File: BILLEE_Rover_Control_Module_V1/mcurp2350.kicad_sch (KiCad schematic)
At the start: 53 parts, among them CN14 DF11-18DP-2DSA, J1 2.54mm Header, SW2 KMR2, SW3 RESET SW, U15 W25Q128JVSIQTR, U16 SN74LVC244APWR, U17 ABM8-272-T3_C20625731, U18 RP2350A_C42411118, U21 TCA4307DGKR, U22 TCA4307DGKR

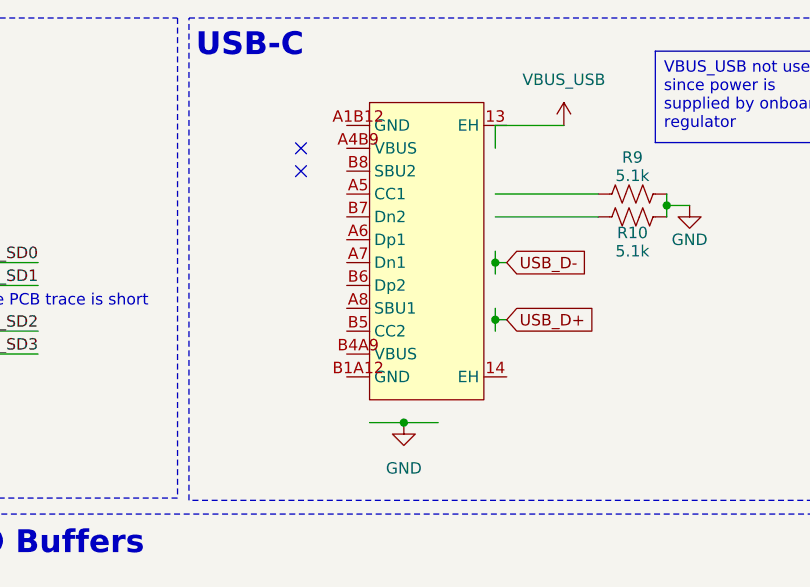
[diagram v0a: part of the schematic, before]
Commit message: Updated for schematic review by claude
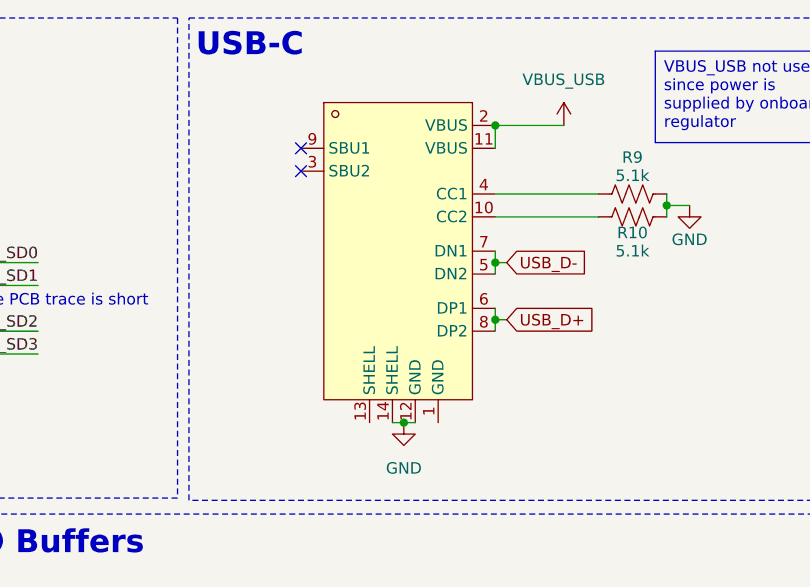
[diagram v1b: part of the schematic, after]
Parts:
- removed USB1: TYPE-C 16PIN 2MD, PDB_LCSC:USB-C-SMD_TYPE-C-16PIN-2MD-073, symbol PDB_LCSC_Libs:TYPE-C16PIN2MD
- added USB2: TYPE-C 16PIN 2MD, PDB_LCSC:USB-C-SMD_TYPE-C-16PIN-2MD-073, symbol PDB_LCSC_Libs:TYPE-C16PIN2MD
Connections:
- net GND: now also USB2.12 (GND), USB2.14 (SHELL)
- net USB_D+: now also USB2.6 (DP1), USB2.8 (DP2)
- net USB_D-: now also USB2.5 (DN2), USB2.7 (DN1)
- net VBUS_USB: now also USB2.11 (VBUS), USB2.2 (VBUS)
- net at R9.1: now also USB2.4 (CC1)
- net at R10.1: now also USB2.10 (CC2)
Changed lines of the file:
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@@
 	)
 	(junction
+		(at 363.22 26.67)
+		(diameter 0)
+		(color 0 0 0 0)
+	)
+	(junction
 		(at 99.06 46.99)
 		(diameter 0)
@@
 	(wire
 		(pts
-			(xy 353.06 59.69) (xy 356.87 59.69)
+			(xy 353.06 59.69) (xy 354.33 59.69)
 		)
 		(stroke
@@
 	(wire
 		(pts
+			(xy 351.79 59.69) (xy 353.06 59.69)
+		)
+		(stroke
+			(width 0)
+			(type default)
+		)
+	)
+	(wire
+		(pts
 			(xy 153.67 123.19) (xy 154.94 123.19)
 		)
@@
 	(wire
 		(pts
-			(xy 349.25 59.69) (xy 353.06 59.69)
-		)
-		(stroke
-			(width 0)
-			(type default)
-		)
-	)
-	(wire
-		(pts
 			(xy 67.31 68.58) (xy 31.75 68.58)
 		)
@@
 	)
 	(symbol
+		(lib_name "TYPE-C16PIN2MD_1")
+		(lib_id "PDB_LCSC_Libs:TYPE-C16PIN2MD")
+		(at 353.06 40.64 0)
+		(unit 1)
+		(body_style 1)
+		(exclude_from_sim no)
+		(in_bom yes)
+		(on_board yes)
+		(in_pos_files yes)
+		(dnp no)
+		(fields_autoplaced yes)
+		(property "Reference" "USB2"
+			(at 353.06 21.59 0)
+			(hide yes)
+			(show_name no)
+			(do_not_autoplace no)
+			(effects
+				(font
+					(size 1.27 1.27)
+				)
+			)
+		)
+		(property "Value" "TYPE-C 16PIN 2MD"
+			(at 353.06 59.69 0)
+			(hide yes)
+			(show_name no)
+			(do_not_autoplace no)
+			(effects
+				(font
+					(size 1.27 1.27)
+				)
+			)
+		)
+		(property "Footprint" "PDB_LCSC:USB-C-SMD_TYPE-C-16PIN-2MD-073"
+			(at 353.06 62.23 0)
+			(hide yes)
+			(show_name no)
+			(do_not_autoplace no)
+			(effects
+				(font
+					(size 1.27 1.27)
+				)
+			)
+		)
+		(property "Datasheet" "https://www.lcsc.com/datasheet/C2765186.pdf"
+			(at 353.06 64.77 0)
+			(hide yes)
+			(show_name no)
+			(do_not_autoplace no)
+			(effects
+				(font
+					(size 1.27 1.27)
+				)
+			)
+		)
+		(property "Description" ""
+			(at 353.06 40.64 0)
+			(hide yes)
+			(show_name no)
+			(do_not_autoplace no)
+			(effects
+				(font
+					(size 1.27 1.27)
+				)
+			)
+		)
+		(property "Manufacturer" "SHOU HAN(首韩)"
+			(at 353.06 67.31 0)
+			(hide yes)
+			(show_name no)
+			(do_not_autoplace no)
+			(effects
+				(font
+					(size 1.27 1.27)
+				)
+			)
+		)
+		(property "MPN" "TYPE-C 16PIN 2MD(073)"
+			(at 353.06 69.85 0)
+			(hide yes)
+			(show_name no)
+			(do_not_autoplace no)
+			(effects
+				(font
+					(size 1.27 1.27)
+				)
+			)
+		)
+		(property "LCSC Part" "C2765186"
+			(at 353.06 72.39 0)
+			(hide yes)
+			(show_name no)
+			(do_not_autoplace no)
+			(effects
+				(font
+					(size 1.27 1.27)
+				)
+			)
+		)
+		(pin "2"
+		)
+		(pin "9"
+		)
+		(pin "13"
+		)
+		(pin "14"
+		)
+		(pin "4"
+		)
+		(pin "1"
+		)
+		(pin "5"
+		)
+		(pin "3"
+		)
+		(pin "6"
+		)
+		(pin "7"
+		)
+		(pin "8"
+		)
+		(pin "11"
+		)
+		(pin "10"
+		)
+		(pin "12"
+		)
+		(instances
+			(project "BILLEE_Rover_Control_Module_V1"
+				(path "/e701dc98-f022-461d-84b5-6b2dd8d89d58/46ee40fa-f724-4b58-ad1f-c10301d1abb5"
+					(reference "USB2")
+					(unit 1)
+				)
+			)
+		)
+	)
+	(symbol
 		(lib_id "Device:R_US")
 		(at 363.22 95.25 180)
@@
 					(unit 1)
 				)
-			)
-		)
-	)
-	(symbol
-		(lib_id "PDB_LCSC_Libs:TYPE-C16PIN2MD")
-		(at 353.06 40.64 0)
-		(unit 1)
-		(body_style 1)
-		(exclude_from_sim no)
-		(in_bom yes)
-		(on_board yes)
-		(in_pos_files yes)
-		(dnp no)
-		(fields_autoplaced yes)
-		(property "Reference" "USB1"
-			(at 353.06 21.59 0)
-			(hide yes)
-			(show_name no)
-			(do_not_autoplace no)
-			(effects
-				(font
-					(size 1.27 1.27)
-				)
-			)
-		)
-		(property "Value" "TYPE-C 16PIN 2MD"
-			(at 353.06 59.69 0)
-			(hide yes)
-			(show_name no)
-			(do_not_autoplace no)
-			(effects
-				(font
-					(size 1.27 1.27)
-				)
-			)
-		)
-		(property "Footprint" "PDB_LCSC:USB-C-SMD_TYPE-C-16PIN-2MD-073"
-			(at 353.06 62.23 0)
-			(hide yes)
-			(show_name no)
-			(do_not_autoplace no)
-			(effects
-				(font
-					(size 1.27 1.27)
-				)
-			)
-		)
-		(property "Datasheet" "https://www.lcsc.com/datasheet/C2765186.pdf"
-			(at 353.06 64.77 0)
-			(hide yes)
-			(show_name no)
-			(do_not_autoplace no)
-			(effects
-				(font
-					(size 1.27 1.27)
-				)
-			)
-		)
-		(property "Description" ""
-			(at 353.06 40.64 0)
-			(hide yes)
-			(show_name no)
-			(do_not_autoplace no)
-			(effects
-				(font
-					(size 1.27 1.27)
-				)
-			)
-		)
-		(property "Manufacturer" "SHOU HAN(首韩)"
-			(at 353.06 67.31 0)
-			(hide yes)
-			(show_name no)
-			(do_not_autoplace no)
-			(effects
-				(font
-					(size 1.27 1.27)
-				)
-			)
-		)
-		(property "MPN" "TYPE-C 16PIN 2MD(073)"
-			(at 353.06 69.85 0)
-			(hide yes)
-			(show_name no)
-			(do_not_autoplace no)
-			(effects
-				(font
-					(size 1.27 1.27)
-				)
-			)
-		)
-		(property "LCSC Part" "C2765186"
-			(at 353.06 72.39 0)
-			(hide yes)
-			(show_name no)
-			(do_not_autoplace no)
-			(effects
-				(font
-					(size 1.27 1.27)
-				)
-			)
-		)
-		(pin "A6"
-		)
-		(pin "A4B9"
-		)
-		(pin "A1B12"
-		)
-		(pin "B5"
-		)
-		(pin "B8"
-		)
-		(pin "13"
-		)
-		(pin "B1A12"
-		)
-		(pin "A5"
-		)
-		(pin "A7"
-		)
-		(pin "B4A9"
-		)
-		(pin "A8"
-		)
-		(pin "B6"
-		)
-		(pin "B7"
-		)
-		(pin "14"
-		)
-		(instances
-			(project "BILLEE_Rover_Control_Module_V1"
-				(path "/e701dc98-f022-461d-84b5-6b2dd8d89d58/46ee40fa-f724-4b58-ad1f-c10301d1abb5"
-					(reference "USB1")
-					(unit 1)
-				)
